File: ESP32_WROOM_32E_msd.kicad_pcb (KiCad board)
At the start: 2 copper layers, 49.5 x 74 mm, 21 parts, among them J1 XH_6pin, J2 XH_6pin, J3 XH_2pin, J5 Conn_01x04_Socket, SW1 SW_SPDT, U2 MCP2561-E-SN

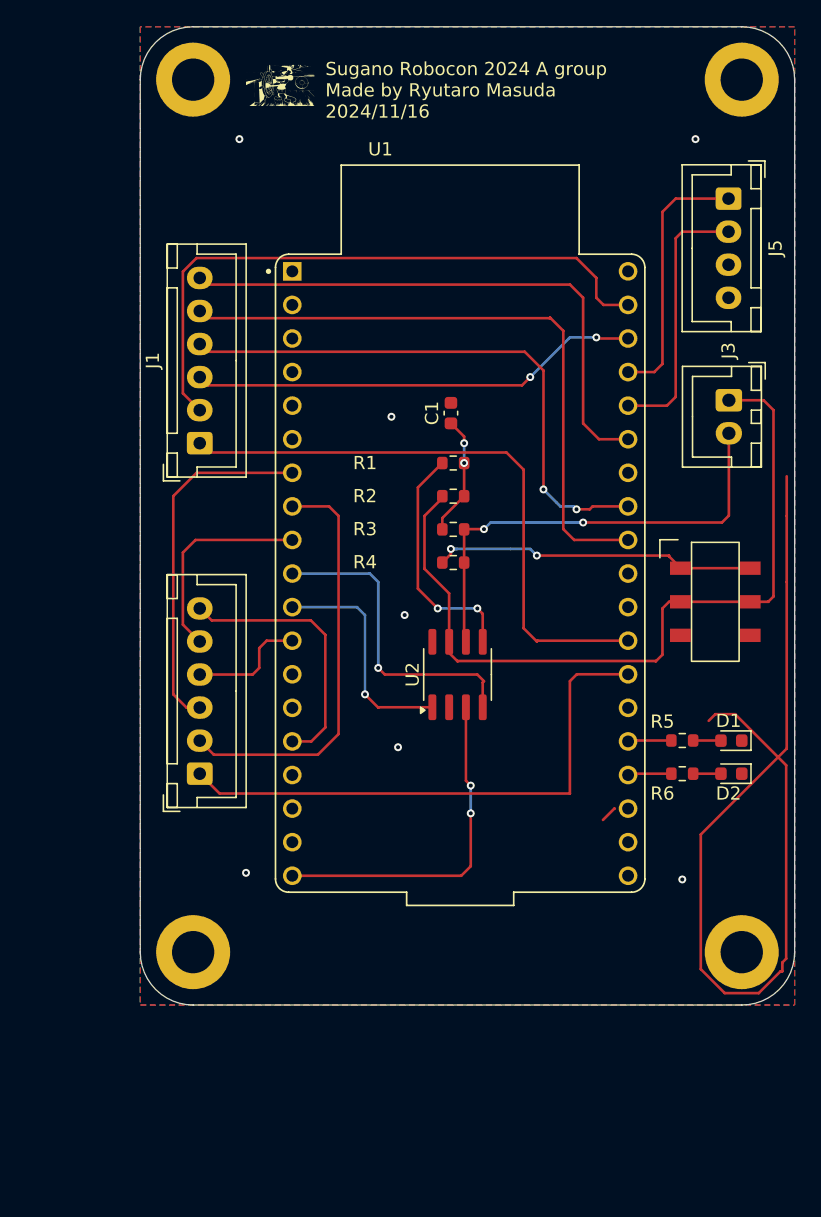
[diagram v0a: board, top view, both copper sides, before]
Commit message: almost complete
add Beta Ground,
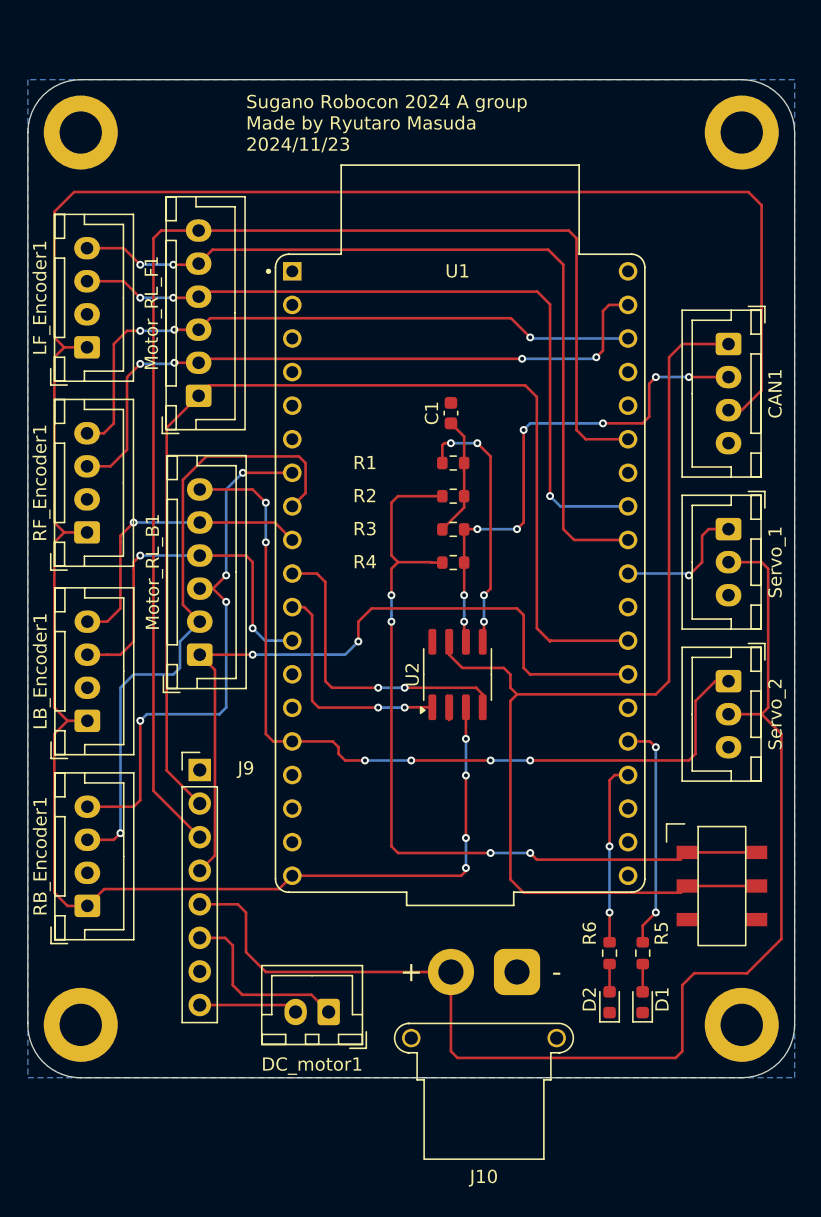
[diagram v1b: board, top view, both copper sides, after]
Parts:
- removed G***: LOGO, my_library:mickey
- removed J3: XH_2pin, Connector_JST:JST_XH_B2B-XH-A_1x02_P2.50mm_Vertical
- added DC_motor1: DC_Motor, Connector_JST:JST_XH_B2B-XH-A_1x02_P2.50mm_Vertical, F.Cu at (100.2, 111.5)
- added J10: 7.5V, Connector_AMASS:AMASS_XT30PW-F_1x02_P2.50mm_Horizontal, F.Cu at (114.5, 108.5)
- added J9: Motor_Driver, Connector_PinHeader_2.54mm:PinHeader_1x08_P2.54mm_Vertical, F.Cu at (90.5, 93.2)
- added LB_Encoder1: LB_Encoder, Connector_JST:JST_XH_B4B-XH-A_1x04_P2.50mm_Vertical, F.Cu at (82.0, 89.5)
- added LF_Encoder1: LF_Encoder, Connector_JST:JST_XH_B4B-XH-A_1x04_P2.50mm_Vertical, F.Cu at (82.0, 61.2)
- added RB_Encoder1: RB_Encoder, Connector_JST:JST_XH_B4B-XH-A_1x04_P2.50mm_Vertical, F.Cu at (82.0, 103.5)
- added RF_Encoder1: RF_Encoder, Connector_JST:JST_XH_B4B-XH-A_1x04_P2.50mm_Vertical, F.Cu at (82.0, 75.2)
- added Servo_1: Servo_1, Connector_JST:JST_XH_B3B-XH-A_1x03_P2.50mm_Vertical, F.Cu at (130.5, 75.0)
- added Servo_2: Servo_2, Connector_JST:JST_XH_B3B-XH-A_1x03_P2.50mm_Vertical, F.Cu at (130.5, 86.5)
- CAN1: renamed from J5; value Conn_01x04_Socket -> CAN_External_Pin
- Motor_RL_B1: renamed from J2; value XH_6pin -> Motor_RL_B
- Motor_RL_F1: renamed from J1; value XH_6pin -> Motor_RL_F
- moved SW1 21.5 mm to (130.0, 102.0)
- moved D1 20.9 mm to (124.0, 110.8), turned to 90 degrees
- moved D2 19.6 mm to (121.5, 110.8), turned to 90 degrees
- moved R5 16.4 mm to (124.0, 107.1), turned to -90 degrees
- moved R6 14.6 mm to (121.5, 107.1), turned to -90 degrees
- moved CAN1 11.0 mm to (130.5, 61.0)
- moved H1 10.1 mm to (81.5, 112.5)
- moved H3 9.39 mm to (81.5, 45.0)
- moved Motor_RL_B1 9.00 mm to (90.5, 84.5)
- moved H2 5.50 mm to (131.5, 112.5)
- moved H4 4.00 mm to (131.5, 45.0)
- moved Motor_RL_F1 3.58 mm to (90.4, 64.9)
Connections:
- CAN1 pad 1: UART_TX -> CAN_H
- CAN1 pad 2: UART_RX -> CAN_L
- R2 pad 1: CAN_H -> Net-(SW1-A)
- U1 pad J3_10: unconnected-(U1-IO5-PadJ3_10) -> Servo1
- U1 pad J3_4: UART_TX -> unconnected-(U1-TXD0-PadJ3_4)
- U1 pad J3_5: UART_RX -> unconnected-(U1-RXD0-PadJ3_5)
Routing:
- net +5V: track 26.0 -> 175.2 mm, vias 2 -> 4
- net +7.5V: track 0.00 -> 95.3 mm
- net (no net): track 72.2 -> 0.00 mm
- net LF_PWM: track 43.0 -> 97.9 mm
- net LB_PWM: track 20.3 -> 63.9 mm, vias 0 -> 6
- net RF_PWM: track 45.7 -> 84.0 mm
- net Net-(SW1-A): track 25.1 -> 62.1 mm, vias 2 -> 4
- net CAN_H: track 57.8 -> 82.7 mm
- net UART_RX: track 20.1 -> 0.00 mm
- net UART_TX: track 19.8 -> 0.00 mm
- net LB_2: track 8.94 -> 27.7 mm, vias 0 -> 2
- net RB_2: track 31.9 -> 48.1 mm, vias 0 -> 1
- net RB_PWM: track 41.7 -> 56.4 mm, vias 0 -> 2
- net RF_1: track 34.2 -> 48.7 mm, vias 2 -> 3
- net LF_1: track 48.4 -> 62.7 mm, vias 0 -> 2
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- removed copper zone on F.Cu, net GND
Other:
- board size 49.5 x 74 mm -> 58 x 75.5 mm
- board text added: "Sugano Robocon 2024 A group Made by Ryutaro Masuda 2024/11/23"
- board text removed: "Sugano Robocon 2024 A group Made by Ryutaro Masuda 2024/11/16"
